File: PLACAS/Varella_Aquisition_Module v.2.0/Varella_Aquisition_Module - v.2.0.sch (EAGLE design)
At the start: 62 parts, among them IC1 M95M04-DRDW6TP, IC10 ICL7660SCBAZ, IC3 M95M04-DRDW6TP, IC4 M95M04-DRDW6TP, IC9 M95M04-DRDW6TP, U1 FT232RLSSOP, X2 USB-SMD-NS, Y2 FA-20H_16.0000MF10Z-AJ0

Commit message: Add files via upload
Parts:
- added R24, R25: 4,7k, rcl:R-EU_R0805
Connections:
- net +3V3: now also R24.2, R25.2
- net SCL3: now also R24.1
- net SDA3: now also R25.1
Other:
- note added: "1/2"
- note added: "2/2"
- note added: "EESC - USP"
- note added: "João Marcus E. Morais de Assunção"
- note added: "Julho de 2020"
- note added: "Microcontrolador"
- note removed: "Microcontroller"
- moved on the sheet: CODE_UPLOAD-1, CODE_UPLOAD-10, CODE_UPLOAD-2, CODE_UPLOAD-3, CODE_UPLOAD-4, CODE_UPLOAD-5, CODE_UPLOAD-6, CODE_UPLOAD-7, CODE_UPLOAD-8, CODE_UPLOAD-9, IC1, IC3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

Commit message: Add files via upload
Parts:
- removed U$1: UVA_MODULE, Zenith_Breakouts:UVA_MODULE
- removed U$4: UVB_MODULE, Zenith_Breakouts:UVB_MODULE
- removed U$5: UVC_MODULE, Zenith_Breakouts:UVC_MODULE
- added 3V3, 5V: (no value), FaBo-PIN:SMD-JUMPER-2
- added R1, R2, R5, R6: 4,7k, rcl:R-EU_R0805
- added U$6, U$7, U$8: MODULO_UV, Zenith_Breakouts:MODULO_UV
- C1, C11: value 0.1uF -> 100nF
- C20: value 0,1uF -> 100nF
- R19, R20, R22: value 1K -> 1k
- RX2: value Green -> (none)
- TX2: value Red -> (none)
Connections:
- removed net -5V: C38.+, IC10.VOUT, U$5.-5V
- new net V+: 3V3.1, 5V.1, IC10.V+, U$8.4
- new net V-: C38.+, IC10.VOUT, U$8.6
- net +3V3: now also 3V3.2, R1.2, R2.2, R5.2, R6.2, U$6.4, U$7.4; no longer U$1.3V3, U$4.3V3
- net +5V: now also 5V.2; no longer IC10.V+, U$5.+5V
- net GND: now also U$6.5, U$7.5, U$8.5; no longer U$1.GND_0, U$1.GND_1, U$1.GND_2, U$4.GND_0, U$4.GND_1, U$4.GND_2, U$5.GND_0, U$5.GND_1, U$5.GND_2
- net SCL1: now also R5.1, U$6.2; no longer U$1.SCL
- net SCL2: now also R1.1, U$7.2; no longer U$4.SCL
- net SDA1: now also R6.1, U$6.1; no longer U$1.SDA
- net SDA2: now also R2.1, U$7.1; no longer U$4.SDA
- net UVC: now also U$8.3; no longer U$5.UVC
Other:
- note added: "João Marcus Epifanio Morais de Assunção, Júlio Calandrin e Leonardo José Ribeiro Baptistella"
- note removed: "João Marcus E. Morais de Assunção"

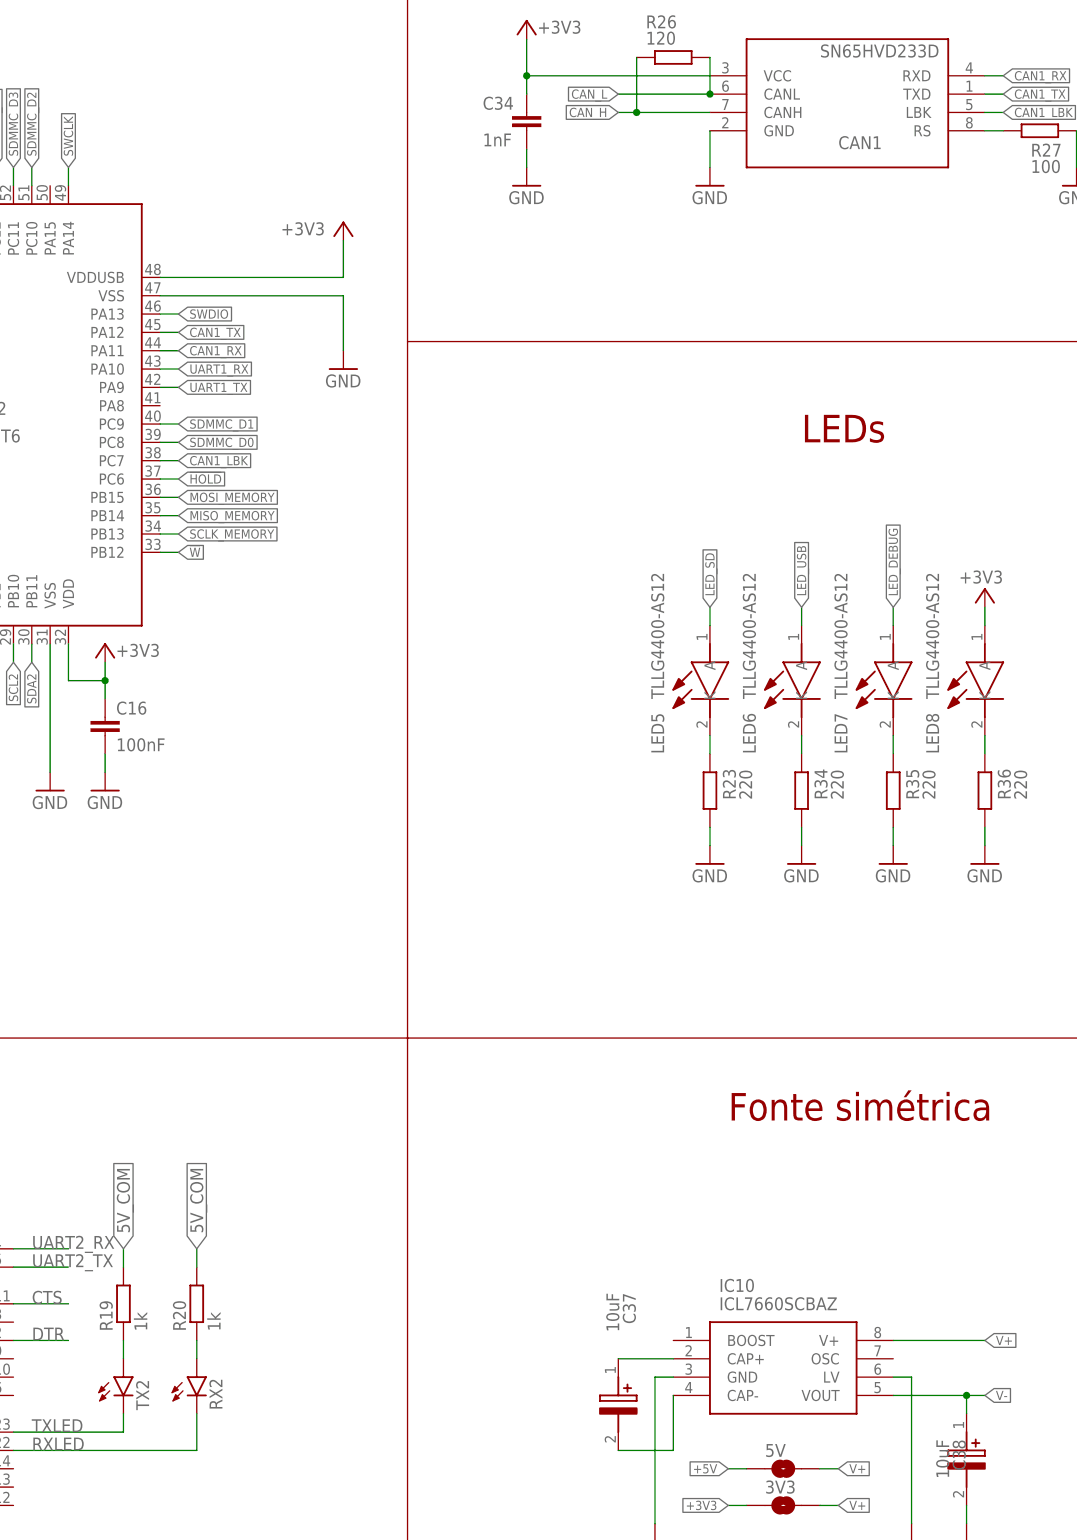
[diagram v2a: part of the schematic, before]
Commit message: Add files via upload
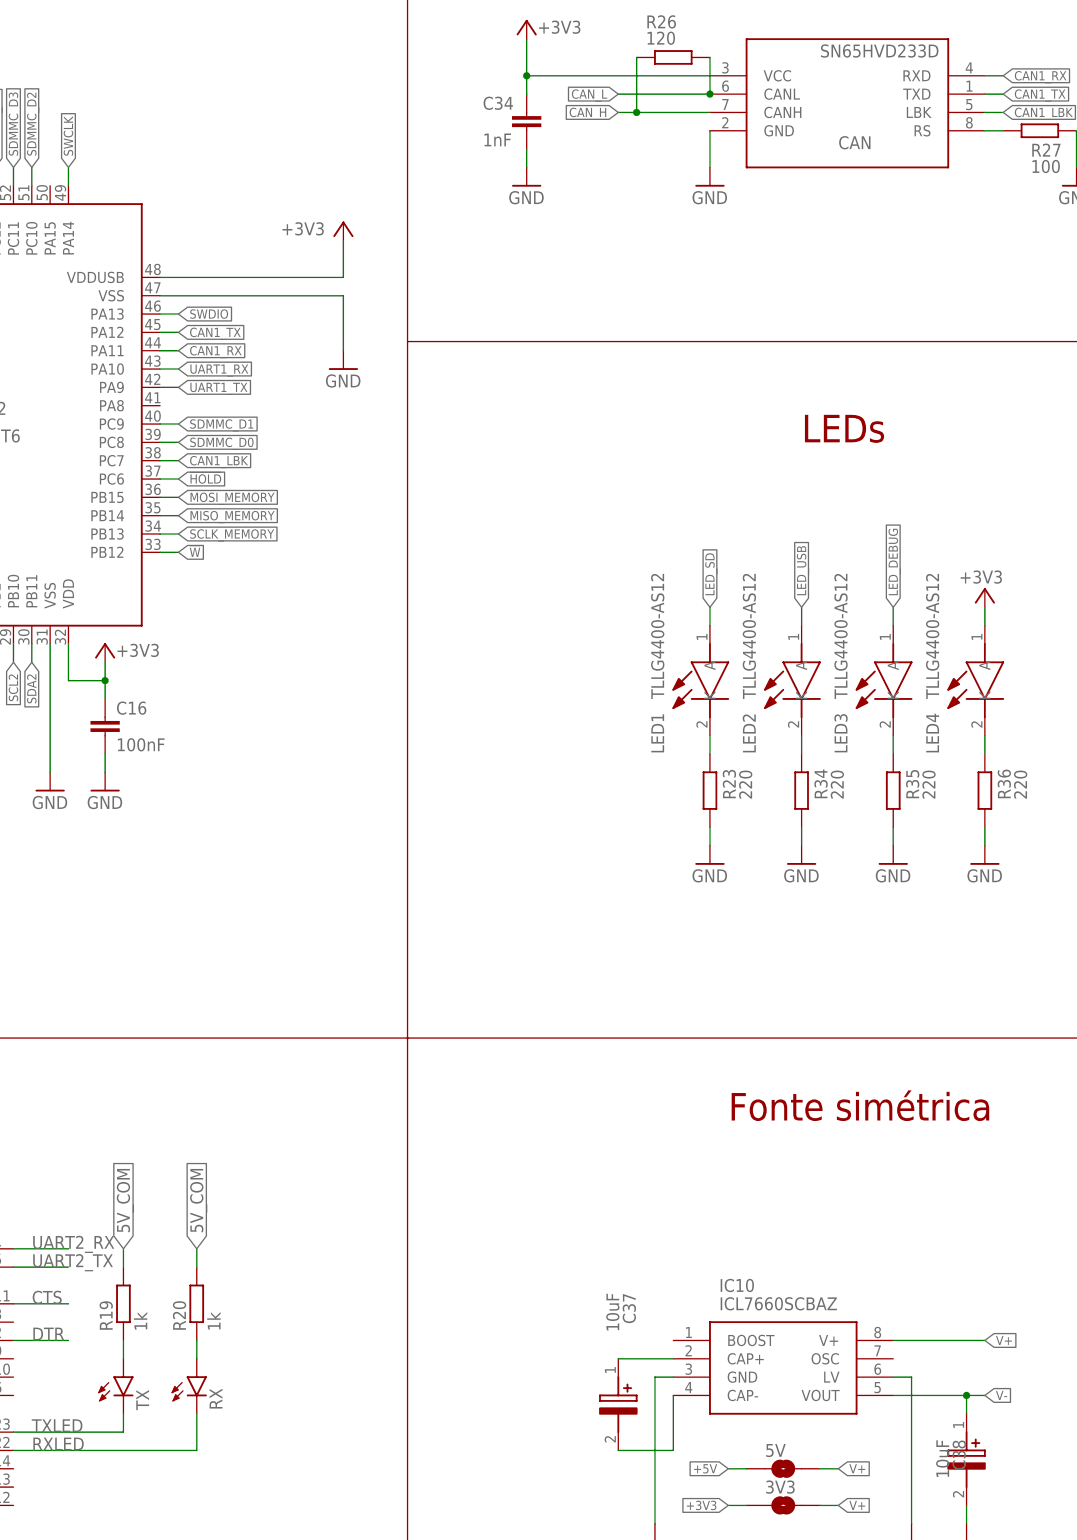
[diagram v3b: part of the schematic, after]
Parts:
- renumbered CAN1 to CAN, LED5 to LED1, LED6 to LED2, LED7 to LED3, LED8 to LED4, RX2 to RX, TX2 to TX
